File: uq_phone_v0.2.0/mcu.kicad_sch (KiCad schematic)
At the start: 40 parts, among them J6 Conn_ARM_SWD_TagConnect_TC2030, J7 559092474, J9 559092474, Q1 MMBT3904LP-7, Q2 MMBT3904LP-7, U17 TXU0204DTRR, U18 TXU0304DTRR, U19 TXU0104DTRR, U20 TXU0104DTRR, U5 TCA9509MRVHR, U6 STM32H723VGHx

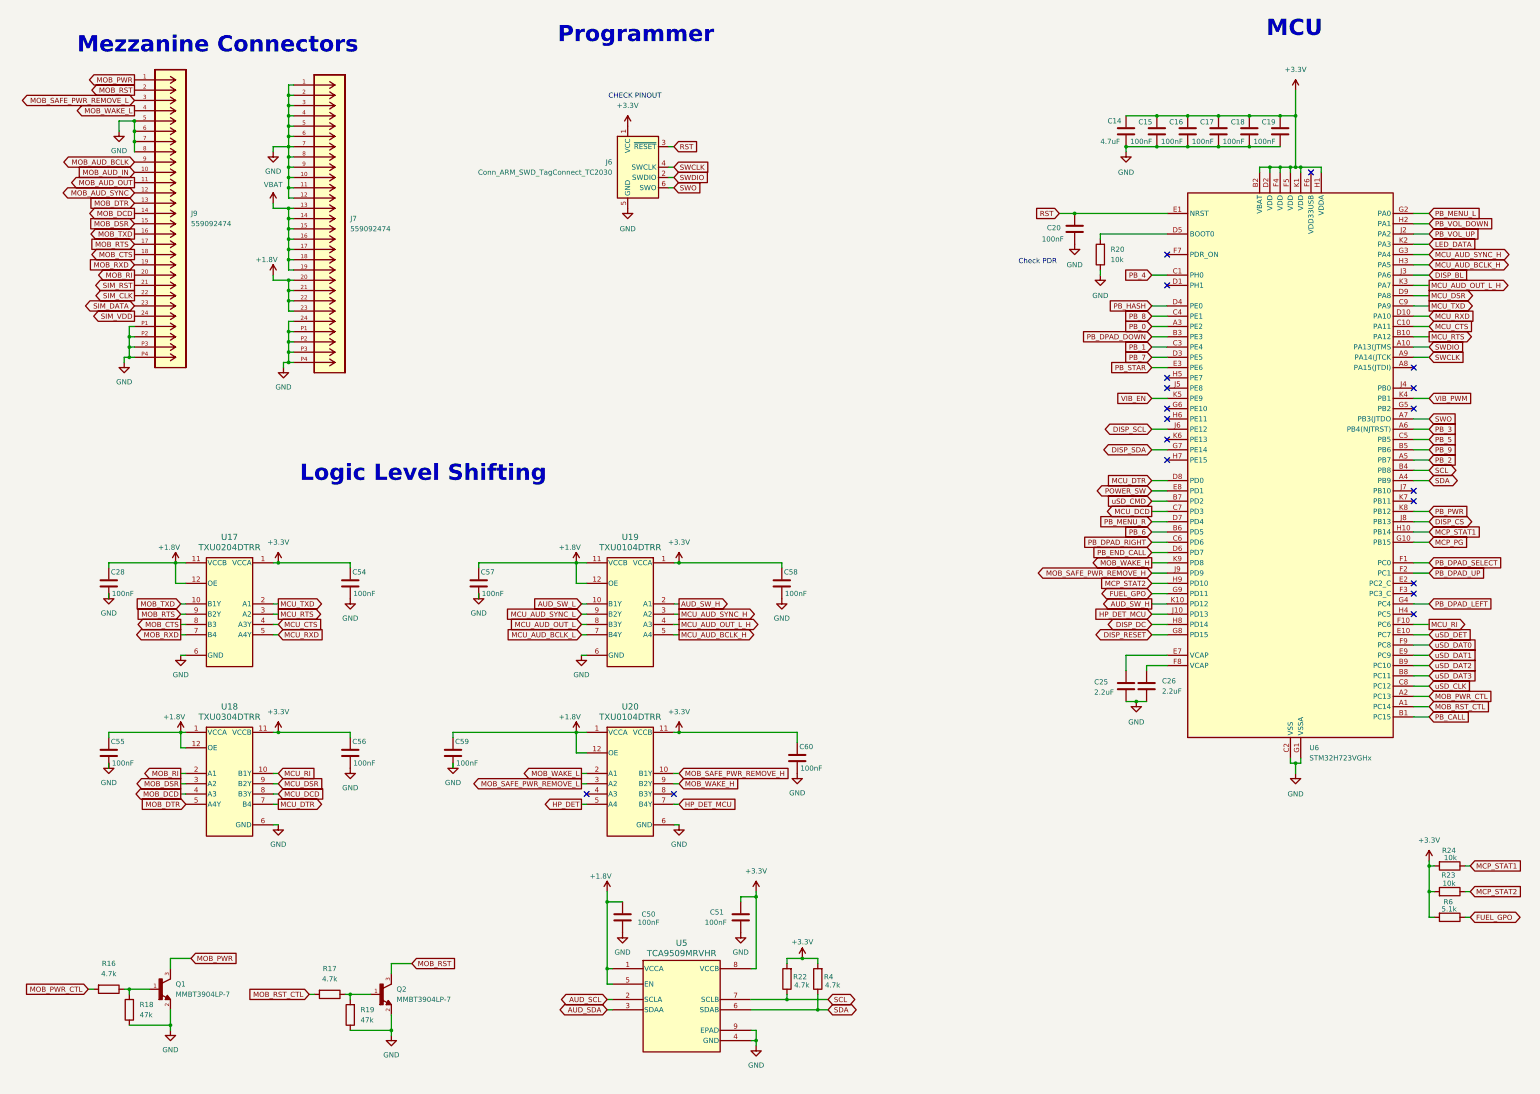
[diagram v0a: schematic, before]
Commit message: Cleaning up adn fixing massive mistake
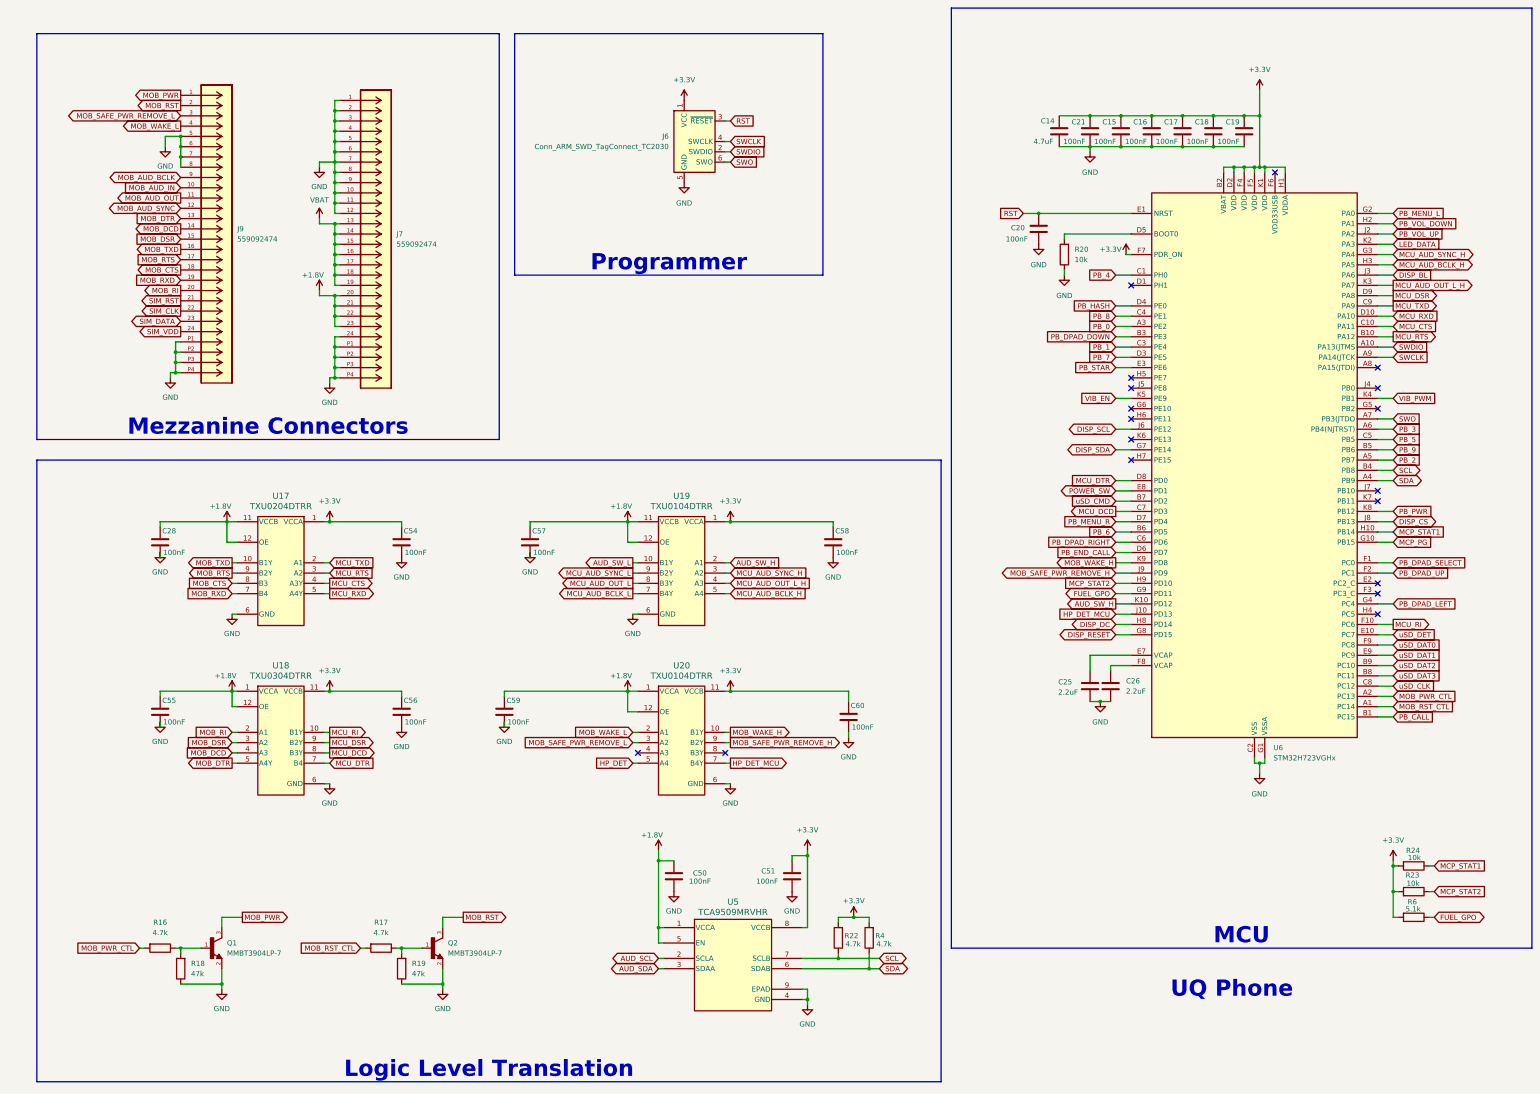
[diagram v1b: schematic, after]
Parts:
- added C21: 100nF, Capacitor_SMD:C_0201_0603Metric, symbol Capacitors:capacitor_100nF
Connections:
- net +3.3V: now also U6.F7 (PDR_ON), C21.2
- net GND: now also C21.1
- net MOB_SAFE_PWR_REMOVE_H: now also U20.9 (B2Y); no longer U20.10 (B1Y)
- net MOB_WAKE_H: now also U20.10 (B1Y); no longer U20.9 (B2Y)
- no-connect marks 19 -> 18
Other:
- note added: "UQ Phone"
- note removed: "CHECK PINOUT"
- note removed: "Check PDR"
- note removed: "Logic Level Shifting"
- note removed: "MCU"
- note removed: "Mezzanine Connectors"
- note removed: "Programmer"
- title: UQ Phone -> Control System
- moved on the sheet: C14, C15, C16, C17, C18, C19, C20, C25, C26, C28, C50, C51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
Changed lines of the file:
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@@
 	(paper "A3")
 	(title_block
-		(title "UQ Phone")
+		(title "Control System")
+		(date "2025-09-05")
 		(rev "0.2.0")
 		(company "The University of Queensland")
+		(comment 1 "James Wood")
 	)
